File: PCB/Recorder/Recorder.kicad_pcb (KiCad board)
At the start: 2 copper layers, 70 x 70 mm, 57 parts, among them J1 Reset, J3 TC2030-USB-NL-DS, J4 TF_PUSH, J5 USB-C-Socket-H, J6 Battery, Q1 CJ2301, SW1 SW_Push_DPDT, U1 ESP32-S3-MINI-1-N4R2, U2 TPS22916CNYFPR, U3 TP4054, U4 ME6211C33M5G-N, U5 ICS-43434, U6 ICS-43434

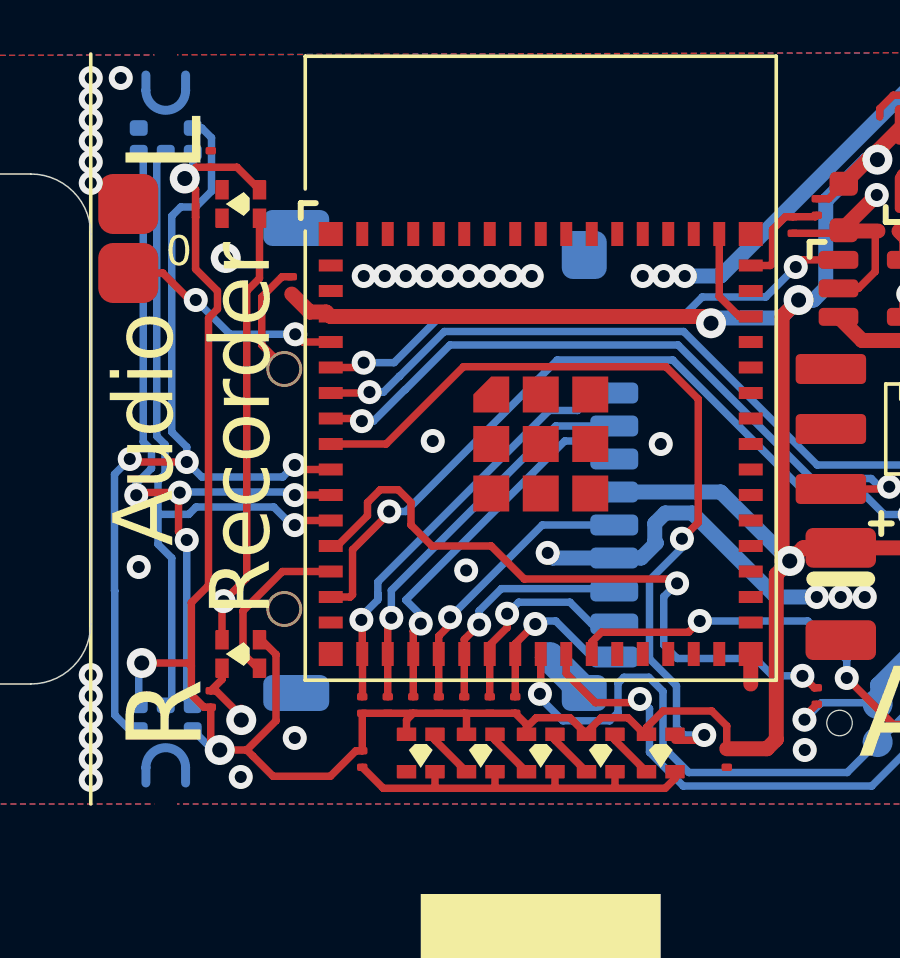
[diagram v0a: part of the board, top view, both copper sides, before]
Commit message: Re render
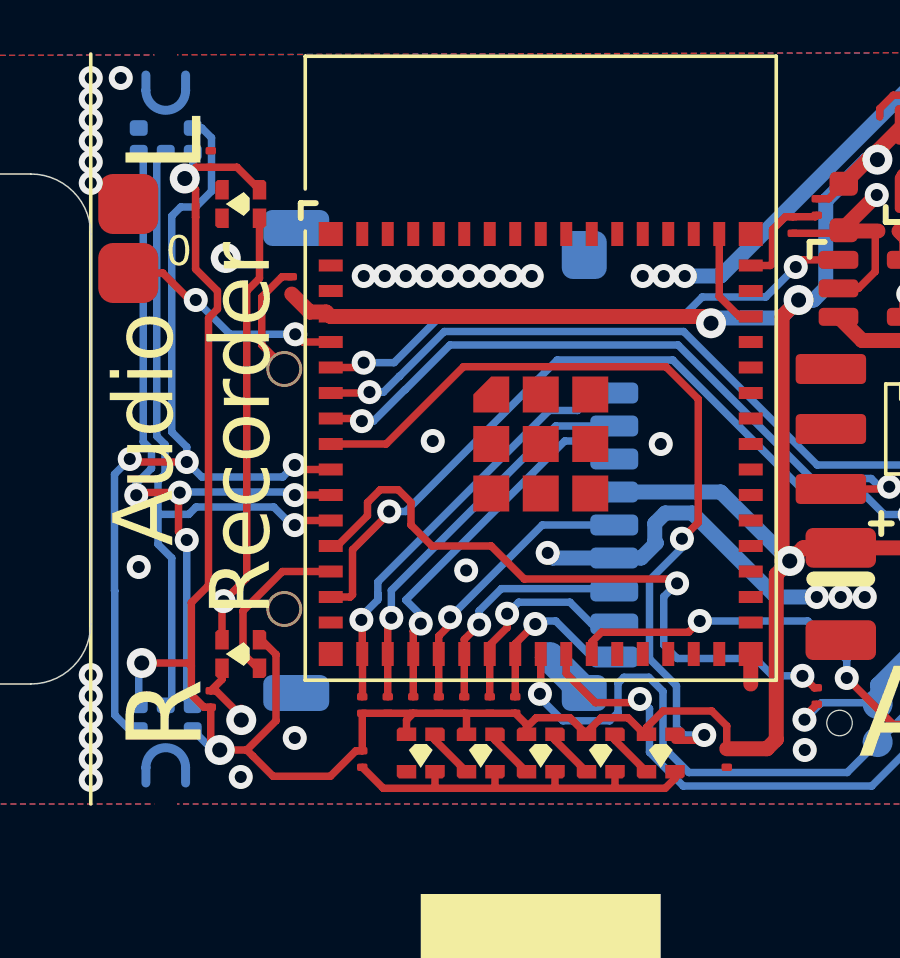
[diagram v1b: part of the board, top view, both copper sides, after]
